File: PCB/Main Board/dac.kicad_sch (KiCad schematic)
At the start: 0 parts

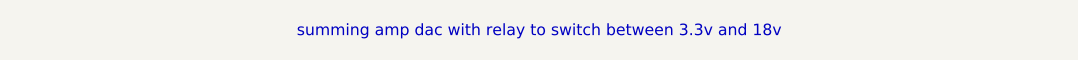
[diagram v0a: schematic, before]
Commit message: minor
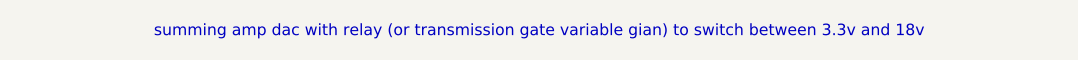
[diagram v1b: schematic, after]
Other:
- note added: "summing amp dac with relay (or transmission gate variable gian) to switch between 3.3v and 18v"
- note removed: "summing amp dac with relay to switch between 3.3v and 18v"
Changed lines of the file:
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@@
 	(generator_version "9.0")
 	(paper "A4")
-	(text "summing amp dac with relay to switch between 3.3v and 18v\n"
+	(text "summing amp dac with relay (or transmission gate variable gian) to switch between 3.3v and 18v\n"
 		(exclude_from_sim no)
 		(at 118.11 80.01 0)

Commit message: beep beep
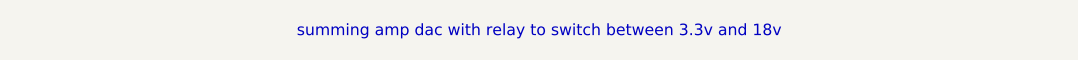
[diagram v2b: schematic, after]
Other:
- note added: "summing amp dac with relay to switch between 3.3v and 18v"
- note removed: "summing amp dac with relay (or transmission gate variable gian) to switch between 3.3v and 18v"
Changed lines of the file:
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@@
 	(generator_version "9.0")
 	(paper "A4")
-	(text "summing amp dac with relay (or transmission gate variable gian) to switch between 3.3v and 18v\n"
+	(text "summing amp dac with relay to switch between 3.3v and 18v\n"
 		(exclude_from_sim no)
 		(at 118.11 80.01 0)
